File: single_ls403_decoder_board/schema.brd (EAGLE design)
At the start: 103.8 x 92.7 mm, 40 parts, among them CON1 LS403_INPUT_CONNECTOR, CON2 CONNECTOR_10PINGENERIC2X5

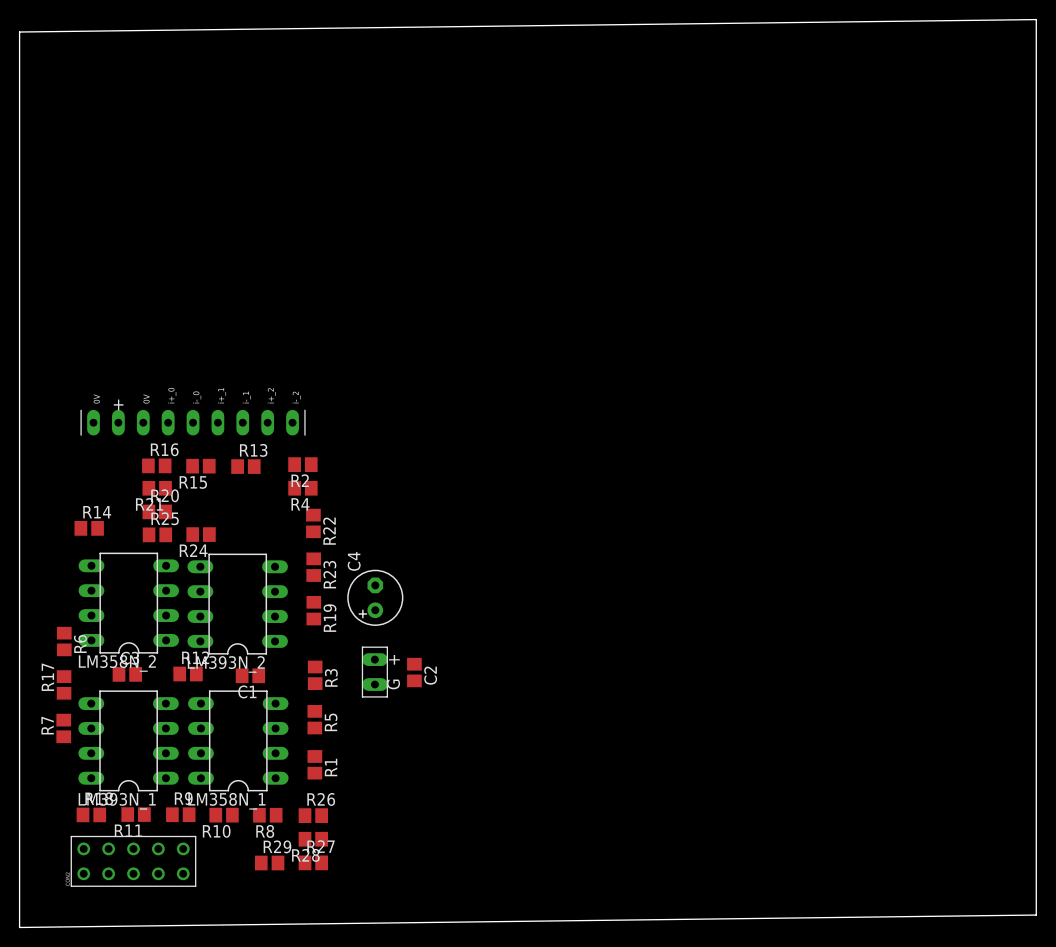
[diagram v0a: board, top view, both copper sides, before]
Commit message: New version of TTL converter ready for batch.
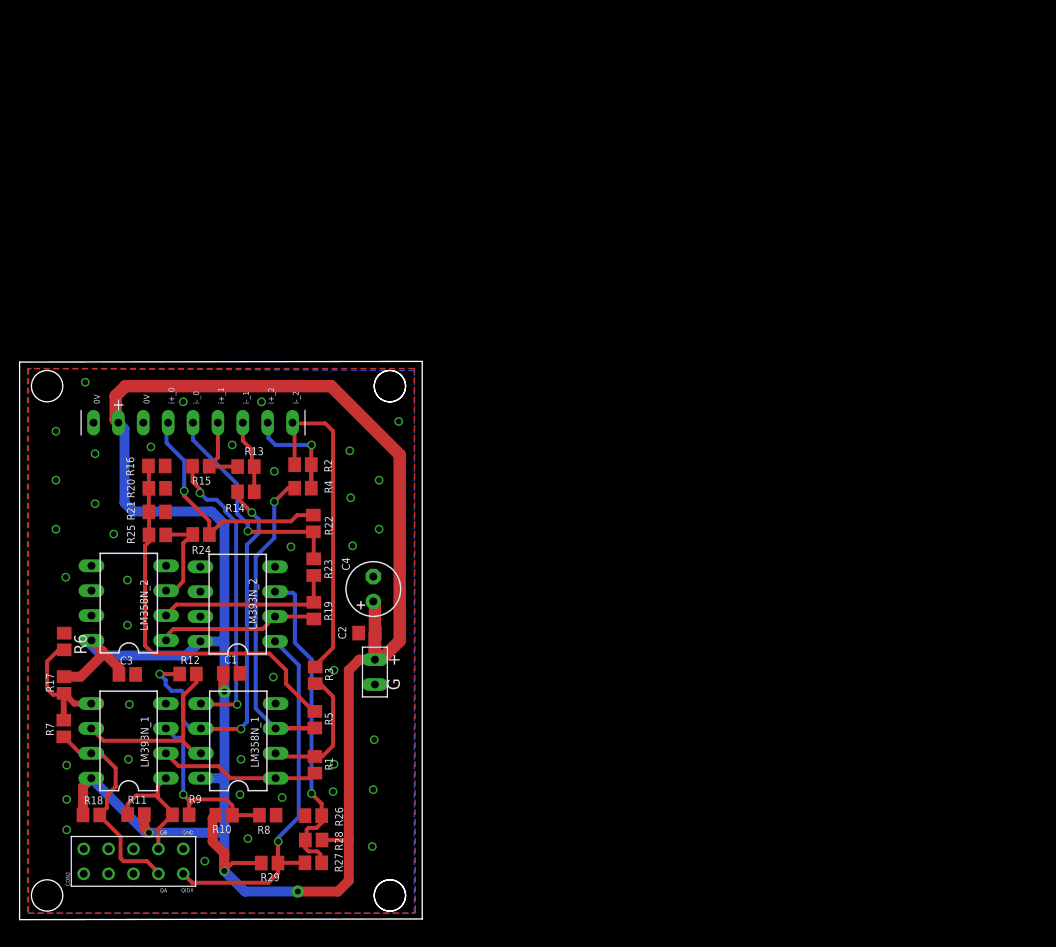
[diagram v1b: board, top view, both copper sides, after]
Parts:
- C4: value (none) -> 22uF
- moved R14 16.4 mm to (19.3, 43.2), turned to 180 degrees
- moved C2 6.31 mm to (31.7, 28.8), turned to 180 degrees
- moved C1 1.93 mm to (17.8, 24.7), turned to 0 degrees
- moved C4 0.92 mm to (32.3, 33.3)
- moved R28 0.09 mm to (26.2, 7.66), turned to 0 degrees
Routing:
- net +5V: track 0.00 -> 224.5 mm, vias 0 -> 4
- net N$8: track 0.00 -> 40.5 mm, vias 0 -> 3
- net VREF: track 0.00 -> 39.5 mm
- net I0_OUT: track 0.00 -> 38.8 mm, vias 0 -> 1
- net N$6: track 0.00 -> 35.3 mm, vias 0 -> 1
- net N$4: track 0.00 -> 33.7 mm
- net N$20: track 0.00 -> 33.0 mm, vias 0 -> 1
- net N$13: track 0.00 -> 30.5 mm, vias 0 -> 2
- net N$18: track 0.00 -> 24.7 mm, vias 0 -> 1
- net N$17: track 0.00 -> 22.9 mm, vias 0 -> 1
- net I1_OUT: track 0.00 -> 22.0 mm
- net N$7: track 0.00 -> 19.8 mm, vias 0 -> 1
- net N$10: track 0.00 -> 19.7 mm
- net N$14: track 0.00 -> 18.4 mm
- net N$3: track 0.00 -> 16.5 mm
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- added copper zone on layer 1, net GND
- added copper zone on layer 16, net GND
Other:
- board size 103.8 x 92.7 mm -> 41.1 x 57 mm
